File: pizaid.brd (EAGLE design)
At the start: 85 x 56 mm, 40 parts

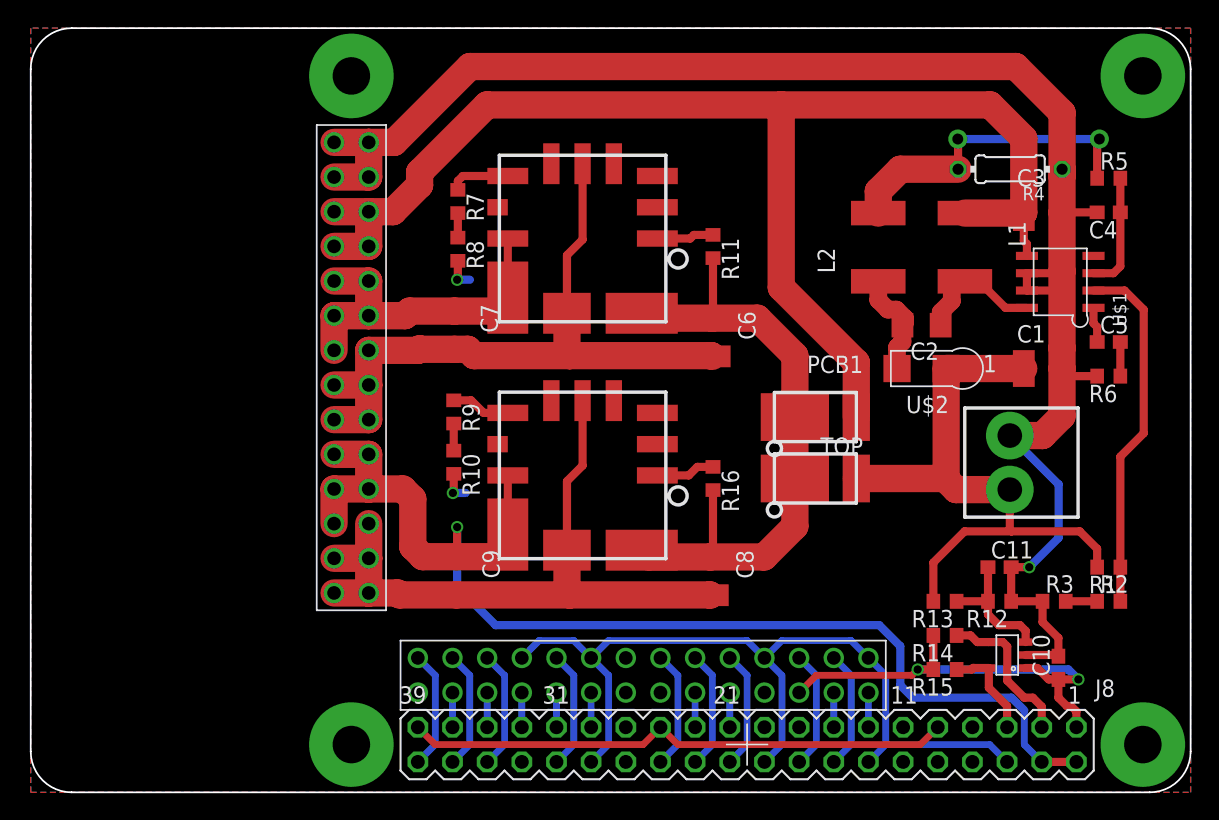
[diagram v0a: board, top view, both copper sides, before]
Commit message: completed rev1
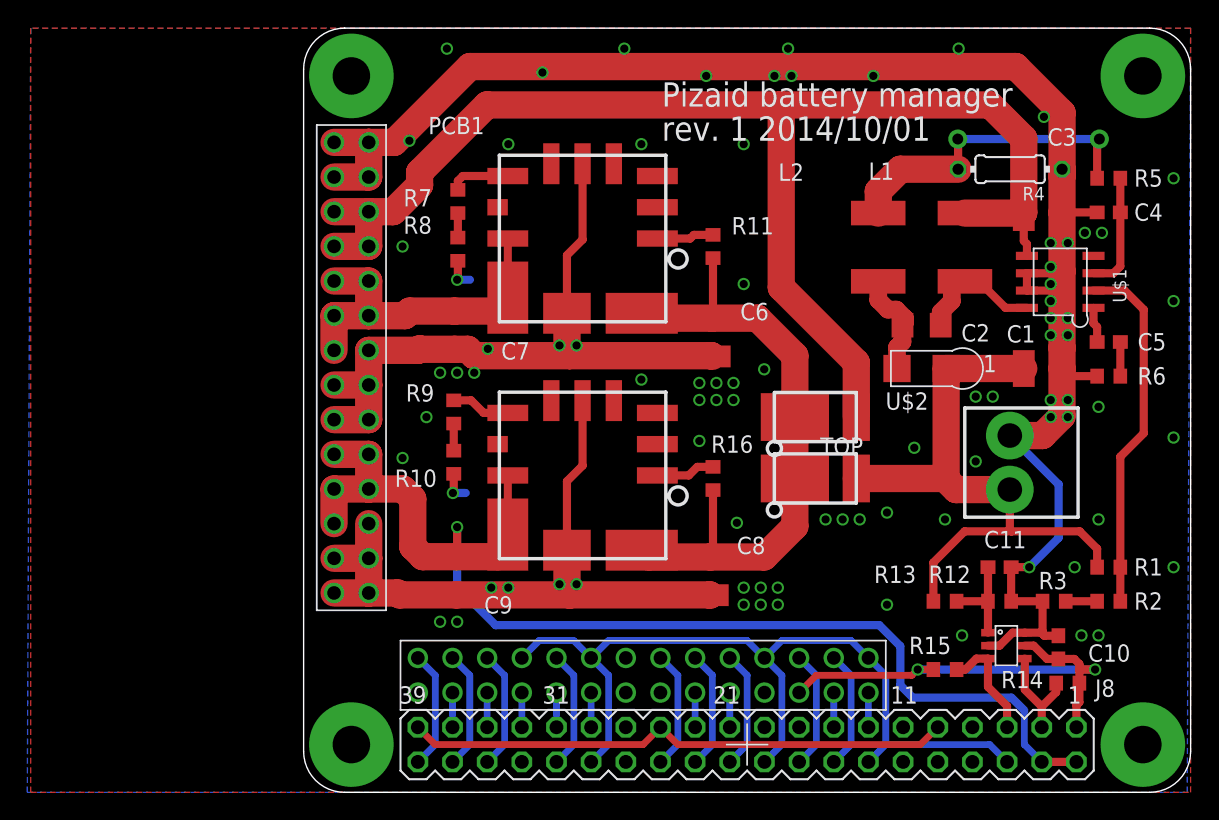
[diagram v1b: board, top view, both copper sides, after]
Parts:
- removed U$16: MCP3021, pizaid:SOT-23
- added U$9: MCP3425, pizaid:SOT-23-6
- moved R14 9.66 mm to (81.0, 12.0), turned to 0 degrees
- moved C10 1.50 mm to (80.3, 14.6)
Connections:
- removed net GND@3: PCB1.25, PCB1.39, PCB1.9
- removed net GND@4: PCB1.14, PCB1.20, PCB1.30, PCB1.34, PCB1.6, U$8.P$1, U$8.P$17, U$8.P$21, U$8.P$7
- net B2: now also U$9.P$5; no longer U$16.P$1
- net GND: now also PCB1.14, PCB1.20, PCB1.25, PCB1.30, PCB1.34, PCB1.39, PCB1.6, PCB1.9, U$8.P$1, U$8.P$17, U$8.P$21, U$8.P$7, U$9.P$2, U$9.P$6; no longer U$16.P$2
- net N$16: now also U$9.P$3; no longer U$16.P$5
- net N$19: now also U$9.P$1; no longer U$16.P$3
- net N$20: now also U$9.P$4; no longer U$16.P$4
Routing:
- net GND: track 232.0 -> 337.2 mm, vias 3 -> 84
- net GND@4: track 64.0 -> 0.00 mm
- net GND@3: track 40.2 -> 0.00 mm
- net N$20: track 11.4 -> 7.70 mm
- net N$19: track 9.85 -> 7.10 mm
- net N$16: track 7.32 -> 8.24 mm
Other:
- board size 85 x 56 mm -> 65 x 56 mm
- board text added: "Pizaid battery manager"
- board text added: "rev. 1 2014/10/01"

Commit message: added gerber
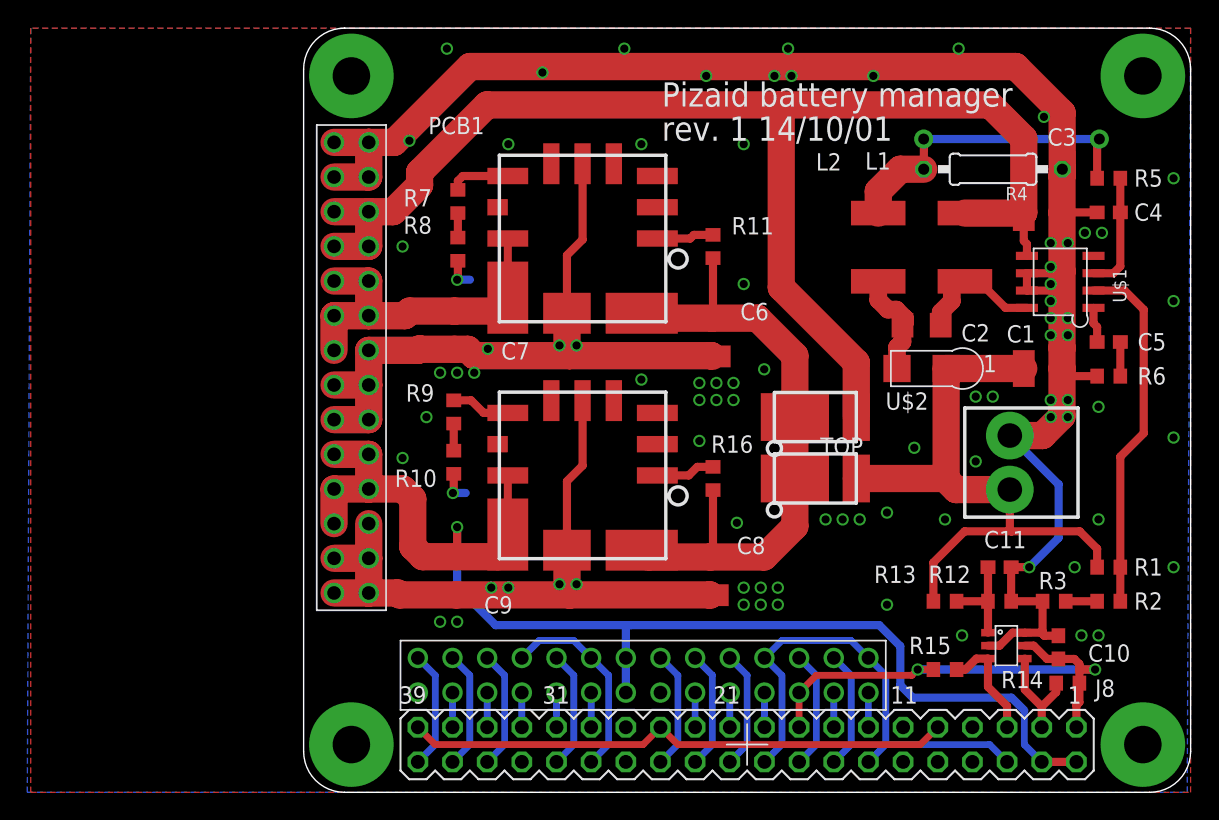
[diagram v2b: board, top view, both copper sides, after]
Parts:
- R4: device rcl:0204/7 -> rcl:0207/10
- moved R4 1.25 mm to (75.5, 49.7)
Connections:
- removed net B7: U$8.P$16
- net 5V0@2: now also U$8.P$15, U$8.P$16
- net B2: now also PCB1.17
- net B3: now also PCB1.19
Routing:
- net GND: track 337.2 -> 323.5 mm
- net 5V0@2: track 91.2 -> 96.2 mm
- net B3: track 0.00 -> 2.54 mm
- net B2: track 34.0 -> 36.5 mm
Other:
- board text added: "rev. 1 14/10/01"
- board text removed: "rev. 1 2014/10/01"
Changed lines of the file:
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@@
 <wire x1="58.75" y1="40.5" x2="64.25" y2="35" width="0.1" layer="42"/>
 <wire x1="64.25" y1="35" x2="64.25" y2="33.75" width="0.1" layer="42"/>
-<wire x1="26" y1="42.5" x2="26" y2="30" width="0.1" layer="42"/>
+<wire x1="26" y1="45.25" x2="26" y2="30" width="0.1" layer="42"/>
 <wire x1="26" y1="30" x2="26" y2="17.5" width="0.1" layer="42"/>
-<wire x1="26" y1="17.5" x2="32" y2="11.5" width="0.1" layer="42"/>
-<wire x1="32" y1="11.5" x2="32" y2="4.25" width="0.1" layer="42"/>
-<wire x1="32" y1="4.25" x2="32" y2="11.5" width="0.1" layer="41"/>
-<wire x1="32" y1="11.5" x2="26" y2="17.5" width="0.1" layer="41"/>
 <wire x1="26" y1="17.5" x2="26" y2="30" width="0.1" layer="41"/>
-<wire x1="26" y1="30" x2="26" y2="42.5" width="0.1" layer="41"/>
+<wire x1="26" y1="30" x2="26" y2="45.25" width="0.1" layer="41"/>
 <wire x1="26" y1="30" x2="35.5" y2="30" width="0.1" layer="42"/>
 <wire x1="35.5" y1="30" x2="40" y2="34.5" width="0.1" layer="42"/>
@@
 <wire x1="25" y1="7" x2="28" y2="4" width="0.1" layer="20" curve="90"/>
 <text x="51.25" y="54.25" size="1.778" layer="21">Pizaid battery manager</text>
-<text x="51.25" y="51.75" size="1.778" layer="21">rev. 1 2014/10/01</text>
+<text x="51.25" y="51.75" size="1.778" layer="21">rev. 1 14/10/01</text>
+<wire x1="31.5" y1="45.25" x2="26" y2="45.25" width="0.1" layer="41"/>
+<wire x1="31.5" y1="45.25" x2="26" y2="45.25" width="0.1" layer="42"/>
 </plain>
 <attributes>
@@
 <attribute name="VALUE" x="78.865" y="21.345" size="1.27" layer="27"/>
 </element>
-<element name="R4" library="rcl" package="0204/7" value="0.2" x="76.77" y="49.6625" smashed="yes" rot="R180">
-<attribute name="NAME" x="79.31" y="48.3671" size="0.9906" layer="25" ratio="10" rot="R180"/>
-<attribute name="VALUE" x="75.6044" y="51.1049" size="0.9906" layer="27" ratio="10"/>
+<element name="R4" library="rcl" package="0207/10" value="0.2" x="75.52" y="49.6625" smashed="yes" rot="R180">
+<attribute name="NAME" x="78.06" y="48.3671" size="0.9906" layer="25" ratio="10" rot="R180"/>
+<attribute name="VALUE" x="74.3544" y="51.1049" size="0.9906" layer="27" ratio="10"/>
 </element>
 <element name="R5" library="rcl" package="R0603" value="24" x="84" y="49" smashed="yes">
@@
 </element>
 <element name="L1" library="rcl" package="L5650M" value="33u" x="73.46" y="43.9475" smashed="yes" rot="R270">
-<attribute name="NAME" x="66.3975" y="48.885" size="1.27" layer="25"/>
-<attribute name="VALUE" x="68.6475" y="49.015" size="1.27" layer="27"/>
+<attribute name="NAME" x="66.1475" y="49.635" size="1.27" layer="25"/>
+<attribute name="VALUE" x="66.1475" y="48.015" size="1.27" layer="27"/>
 </element>
 <element name="L2" library="rcl" package="L5650M" value="33u" x="67.11" y="43.9475" smashed="yes" rot="R90">
-<attribute name="NAME" x="59.7925" y="48.815" size="1.27" layer="25"/>
-<attribute name="VALUE" x="62.5425" y="48.945" size="1.27" layer="27"/>
+<attribute name="NAME" x="62.5425" y="49.565" size="1.27" layer="25"/>
+<attribute name="VALUE" x="62.5425" y="47.945" size="1.27" layer="27"/>
 </element>
 <element name="U$2" library="pizaid" package="SOD-123FL" value="SS2040FL" x="70.285" y="35.0575" smashed="yes" rot="R180">
@@
 <contactref element="U$10" pad="P$2"/>
 <wire x1="80.575" y1="46.4875" x2="80.575" y2="49.1575" width="2" layer="1"/>
-<wire x1="80.575" y1="49.1575" x2="80.58" y2="49.6625" width="2" layer="1"/>
+<wire x1="80.575" y1="49.1575" x2="80.6" y2="49.6625" width="2" layer="1"/>
 <wire x1="80.575" y1="46.4875" x2="80.575" y2="42.1875" width="2" layer="1"/>
 <wire x1="80.575" y1="42.1875" x2="80.575" y2="36.5625" width="2" layer="1"/>
@@
 <wire x1="37.1875" y1="57.1875" x2="77.1875" y2="57.1875" width="2" layer="1"/>
 <wire x1="77.1875" y1="57.1875" x2="80.58" y2="53.795" width="2" layer="1"/>
-<wire x1="80.58" y1="49.6625" x2="80.58" y2="53.795" width="2" layer="1"/>
+<wire x1="80.6" y1="49.6625" x2="80.58" y2="53.795" width="2" layer="1"/>
 <wire x1="44.2975" y1="39.105" x2="44.38" y2="39.1875" width="0.6" layer="1"/>
 <wire x1="44.38" y1="39.1875" x2="45.4375" y2="39.1875" width="0.6" layer="1"/>
@@
 <wire x1="44.795" y1="15.125" x2="42.265" y2="15.125" width="0.5" layer="16"/>
 <wire x1="40.99" y1="13.85" x2="42.265" y2="15.125" width="0.5" layer="16"/>
-<wire x1="46.07" y1="13.85" x2="47.345" y2="15.125" width="0.5" layer="16"/>
-<wire x1="58.77" y1="13.85" x2="57.495" y2="15.125" width="0.5" layer="16"/>
-<wire x1="57.495" y1="15.125" x2="47.345" y2="15.125" width="0.5" layer="16"/>
 <wire x1="58.77" y1="6.23" x2="60.05" y2="7.51" width="0.5" layer="16"/>
 <wire x1="58.77" y1="13.85" x2="60.05" y2="12.57" width="0.5" layer="16"/>
@@
 <via x="60.75" y="56.5" extent="1-16" drill="0.6"/>
 <via x="79.25" y="53.5" extent="1-16" drill="0.6"/>
-<wire x1="80.58" y1="53.795" x2="79.25" y2="53.5" width="0" layer="19" extent="1-1"/>
-<wire x1="28.5" y1="7.5" x2="33.37" y2="8.77" width="0" layer="19" extent="1-1"/>
 </signal>
 <signal name="VCC">
@@
 <wire x1="67.11" y1="46.4475" x2="67.11" y2="48.0475" width="2" layer="1"/>
 <wire x1="67.11" y1="48.0475" x2="68.725" y2="49.6625" width="2" layer="1"/>
-<wire x1="72.96" y1="49.6625" x2="68.725" y2="49.6625" width="2" layer="1"/>
-<wire x1="72.96" y1="49.6625" x2="72.96" y2="51.8525" width="0.6" layer="1"/>
-<wire x1="72.96" y1="51.8525" x2="72.9375" y2="51.875" width="0.6" layer="1"/>
-<via x="72.9375" y="51.875" extent="1-16" drill="0.8" diameter="1.4"/>
-<wire x1="72.9375" y1="51.875" x2="83.3125" y2="51.875" width="0.6" layer="16"/>
+<wire x1="70.44" y1="49.6625" x2="68.725" y2="49.6625" width="2" layer="1"/>
+<wire x1="70.44" y1="49.6625" x2="70.46" y2="51.6025" width="0.6" layer="1"/>
+<wire x1="70.46" y1="51.6025" x2="70.4375" y2="51.875" width="0.6" layer="1"/>
+<via x="70.4375" y="51.875" extent="1-16" drill="0.8" diameter="1.4"/>
+<wire x1="70.4375" y1="51.875" x2="83.3125" y2="51.875" width="0.6" layer="16"/>
 <via x="83.3125" y="51.875" extent="1-16" drill="0.8" diameter="1.4"/>
 <wire x1="83.15" y1="49" x2="83.15" y2="51.7125" width="0.6" layer="1"/>
@@
 <wire x1="77.8125" y1="10" x2="76.875" y2="10.9375" width="0.6" layer="16"/>
 <wire x1="76.875" y1="10.9375" x2="69.6375" y2="10.9375" width="0.6" layer="16"/>
-<wire x1="67.1875" y1="16.25" x2="39.0625" y2="16.25" width="0.6" layer="16"/>
+<wire x1="67.1875" y1="16.25" x2="49" y2="16.25" width="0.6" layer="16"/>
+<wire x1="48.61" y1="16.25" x2="39.0625" y2="16.25" width="0.6" layer="16"/>
 <wire x1="39.0625" y1="16.25" x2="36.25" y2="19.0625" width="0.6" layer="16"/>
 <wire x1="36.25" y1="19.0625" x2="36.25" y2="23.4375" width="0.6" layer="16"/>
@@
 <wire x1="68.725" y1="11.85" x2="68.725" y2="14.7125" width="0.6" layer="16"/>
 <wire x1="68.725" y1="14.7125" x2="67.1875" y2="16.25" width="0.6" layer="16"/>
+<contactref element="U$8" pad="P$15"/>
+<contactref element="U$8" pad="P$16"/>
+<wire x1="48.61" y1="11.31" x2="48.61" y2="13.85" width="0.6" layer="16"/>
+<wire x1="48.61" y1="13.85" x2="48.61" y2="16.25" width="0.6" layer="16"/>
+<wire x1="48.61" y1="16.25" x2="49" y2="16.25" width="0.6" layer="16"/>
 <wire x1="39.9625" y1="22.89" x2="40" y2="24.0625" width="0" layer="19" extent="1-1"/>
 </signal>
@@
 <wire x1="83" y1="13" x2="81.85" y2="13" width="0.6" layer="1"/>
 <wire x1="71.15" y1="13" x2="70" y2="13" width="0.5" layer="1"/>
+<contactref element="PCB1" pad="17"/>
+<wire x1="61.31" y1="8.77" x2="61.31" y2="11.31" width="0.5" layer="1"/>
 </signal>
 <signal name="B3">
 <contactref element="U$8" pad="P$8"/>
+<contactref element="PCB1" pad="19"/>
+<wire x1="58.77" y1="8.77" x2="58.77" y2="11.31" width="0.5" layer="16"/>
 </signal>
 <signal name="B6">
 <contactref element="U$8" pad="P$14"/>
 </signal>
-<signal name="B7">
-<contactref element="U$8" pad="P$16"/>
-</signal>
 <signal name="GIRD">
